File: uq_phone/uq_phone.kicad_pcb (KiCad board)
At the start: 4 copper layers, 116.9 x 105 mm, 170 parts, among them J1 USB4105-GF-A, J10 Conn_01x02, J11 FTSH-105-XX-X-DV, J12 Conn_ARM_SWD_TagConnect_TC2030, J2 S3B-PH-SM4-TB_LF__SN_, J3 20279-001E-03, J4 20279-001E-03, J5 KP15B-6S-SF_800_, J7 Conn_01x02, J8 541324562, J9 SJ-3551B-MSMT-TR-67, Q1 MMBT3904, Q2 MMBT3904, SW1 SKTAAAE010, SW2 SKTAAAE010, U1 MCP73871-2CCI_ML, U10 TPD3F303DQDR, U12 MCP1664T-E/OT, U14 TPD8F003DQDR, U15 TS3A5018RSVR, U16 NAU88C22YG, U2 TPS62162DSGR, U3 BQ27441DRZR-G1A, U4 RC7620_1104625, U5 TXB0108RGYR, U6 TXB0108RGYR, U7 STM32H730VBTx, U8 LSM6DSVTR, U9 DRV2603RUNR

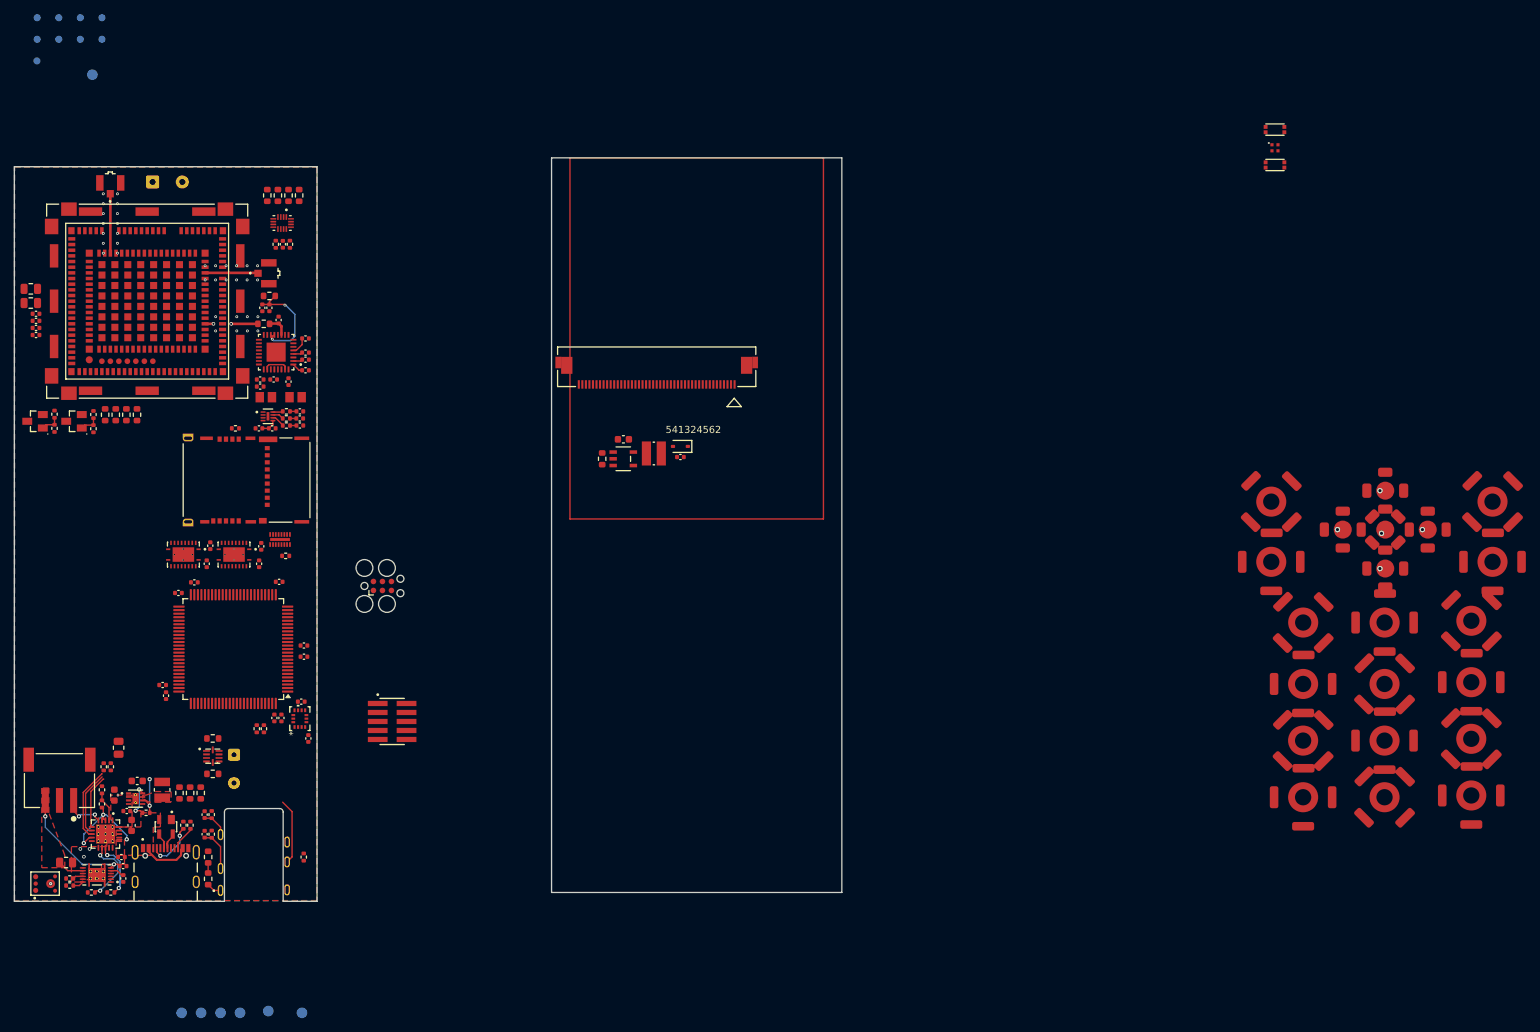
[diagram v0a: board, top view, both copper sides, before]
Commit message: Routing Init
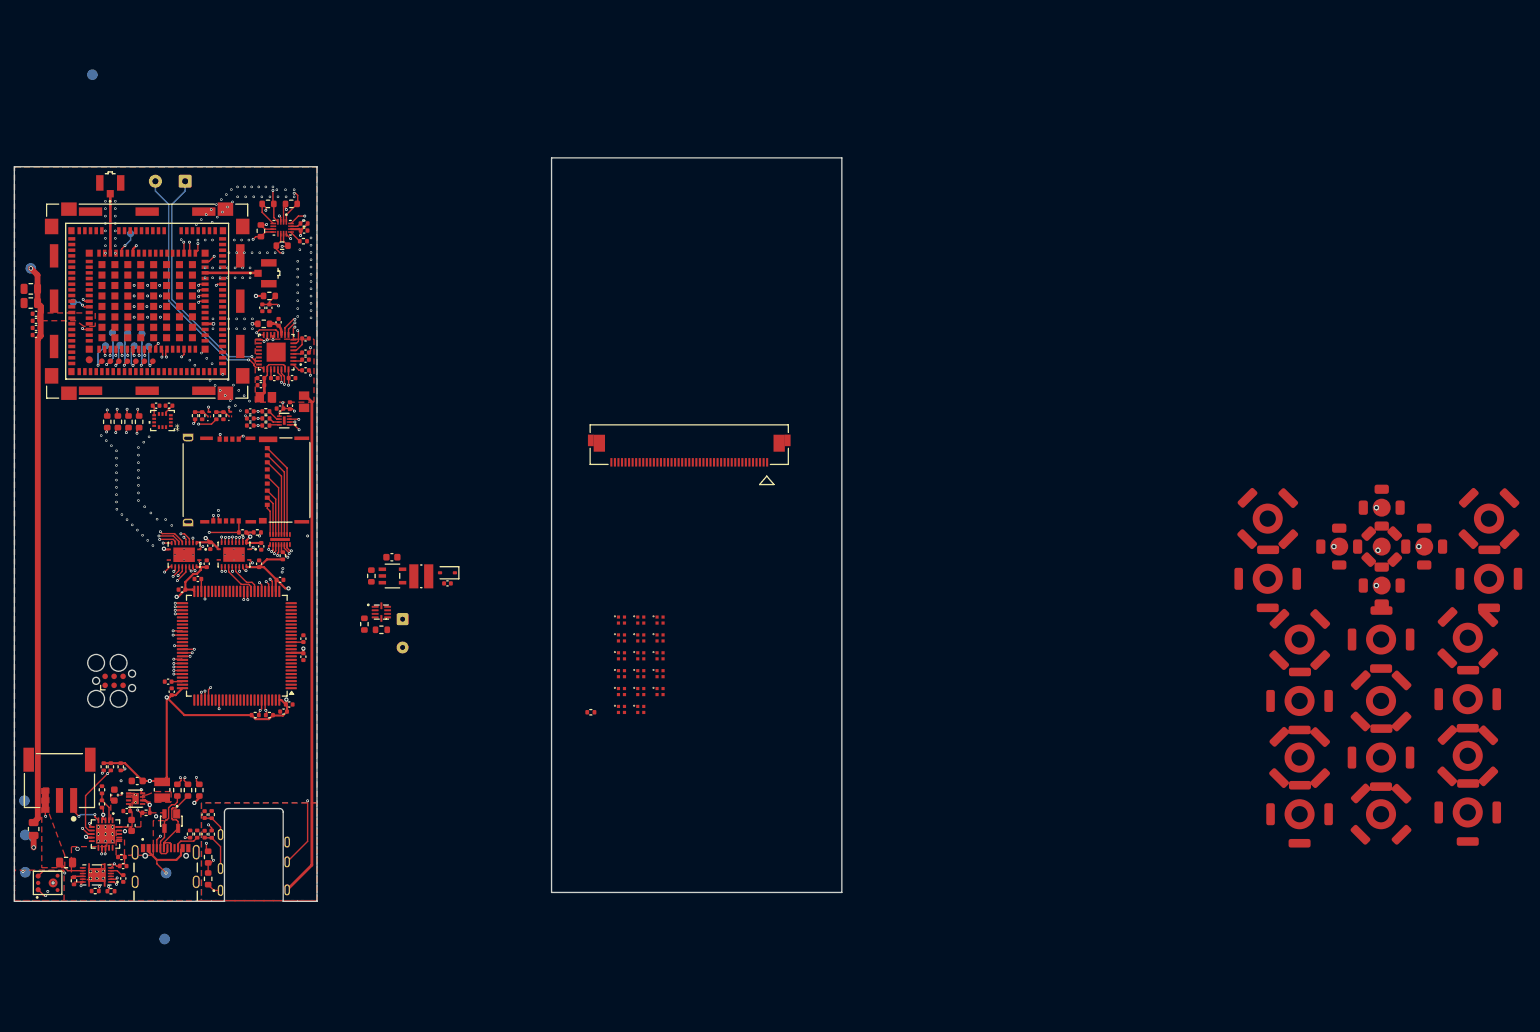
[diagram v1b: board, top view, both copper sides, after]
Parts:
- removed the J11 at (80.7, 146.6)
- removed the REF** at (209.4, 132.6)
- removed the REF** at (236.2, 115.5)
- removed the REF** at (209.4, 149.3)
- removed the REF** at (209.4, 157.3)
- removed the REF** at (209.4, 141.3)
- removed the REF** at (220.9, 149.3)
- removed the REF** at (204.9, 124.0)
- removed the REF** at (215.0, 119.5)
- removed the REF** at (221.0, 114.0)
- removed the REF** at (204.9, 115.5)
- removed the REF** at (220.9, 157.3)
- removed the REF** at (220.9, 141.3)
- removed the REF** at (221.0, 119.5)
- removed the REF** at (233.2, 157.1)
- removed the REF** at (227.0, 119.5)
- removed the REF** at (220.9, 132.6)
- removed the REF** at (233.2, 141.1)
- removed the REF** at (233.2, 132.4)
- removed the REF** at (236.2, 124.0)
- removed the REF** at (233.2, 149.1)
- removed the REF** at (221.0, 125.0)
- removed SW1, SW2: SKTAAAE010, custom_footprints:SKTAAAE010
- added LED10: XL-1010RGBC, custom_footprints:XL-1010RGBC-WS2812B, F.Cu at (115.4, 139.4)
- added LED11: XL-1010RGBC, custom_footprints:XL-1010RGBC-WS2812B, F.Cu at (115.4, 141.9)
- added LED12: XL-1010RGBC, custom_footprints:XL-1010RGBC-WS2812B, F.Cu at (115.4, 144.5)
- added LED13: XL-1010RGBC, custom_footprints:XL-1010RGBC-WS2812B, F.Cu at (118.2, 131.8)
- added LED14: XL-1010RGBC, custom_footprints:XL-1010RGBC-WS2812B, F.Cu at (118.2, 134.4)
- added LED15: XL-1010RGBC, custom_footprints:XL-1010RGBC-WS2812B, F.Cu at (118.2, 136.9)
- added LED16: XL-1010RGBC, custom_footprints:XL-1010RGBC-WS2812B, F.Cu at (118.2, 139.4)
- added LED17: XL-1010RGBC, custom_footprints:XL-1010RGBC-WS2812B, F.Cu at (118.2, 141.9)
- added LED2: XL-1010RGBC, custom_footprints:XL-1010RGBC-WS2812B, F.Cu at (112.7, 134.4)
- added LED3: XL-1010RGBC, custom_footprints:XL-1010RGBC-WS2812B, F.Cu at (112.7, 136.9)
- added LED4: XL-1010RGBC, custom_footprints:XL-1010RGBC-WS2812B, F.Cu at (112.7, 139.4)
- added LED5: XL-1010RGBC, custom_footprints:XL-1010RGBC-WS2812B, F.Cu at (112.7, 141.9)
- added LED6: XL-1010RGBC, custom_footprints:XL-1010RGBC-WS2812B, F.Cu at (112.7, 144.5)
- added LED7: XL-1010RGBC, custom_footprints:XL-1010RGBC-WS2812B, F.Cu at (115.4, 131.8)
- added LED8: XL-1010RGBC, custom_footprints:XL-1010RGBC-WS2812B, F.Cu at (115.4, 134.4)
- added LED9: XL-1010RGBC, custom_footprints:XL-1010RGBC-WS2812B, F.Cu at (115.4, 136.9)
- added R48: 330R, Resistor_SMD:R_0402_1005Metric, F.Cu at (108.8, 145.3)
- added REF**: 8.5mmSnaptron, custom_footprints:8.5mmSnaptron, F.Cu at (220.4, 151.7)
- added REF**: 8.5mmSnaptron, custom_footprints:8.5mmSnaptron, F.Cu at (232.7, 159.4)
- added REF**: 8.5mmSnaptron, custom_footprints:8.5mmSnaptron, F.Cu at (235.7, 118.0)
- added REF**: 8.5mmSnaptron, custom_footprints:8.5mmSnaptron, F.Cu at (232.7, 143.4)
- added REF**: 8.5mmSnaptron, custom_footprints:8.5mmSnaptron, F.Cu at (208.9, 151.7)
- added REF**: 8.5mmSnaptron, custom_footprints:8.5mmSnaptron, F.Cu at (204.4, 118.0)
- added REF**: 8.5mmSnaptron, custom_footprints:8.5mmSnaptron, F.Cu at (232.7, 151.4)
- added REF**: 6mmSnaptron, custom_footprints:6mmSnaptron, F.Cu at (220.5, 127.4)
- added REF**: 8.5mmSnaptron, custom_footprints:8.5mmSnaptron, F.Cu at (220.4, 135.0)
- added REF**: 6mmSnaptron, custom_footprints:6mmSnaptron, F.Cu at (226.5, 121.9)
- added REF**: 6mmSnaptron, custom_footprints:6mmSnaptron, F.Cu at (214.5, 121.9)
- added REF**: 8.5mmSnaptron, custom_footprints:8.5mmSnaptron, F.Cu at (204.4, 126.5)
- added REF**: 6mmSnaptron, custom_footprints:6mmSnaptron, F.Cu at (220.5, 116.4)
- added REF**: 8.5mmSnaptron, custom_footprints:8.5mmSnaptron, F.Cu at (208.9, 135.0)
- added REF**: 8.5mmSnaptron, custom_footprints:8.5mmSnaptron, F.Cu at (220.4, 159.7)
- added REF**: 6mmSnaptron, custom_footprints:6mmSnaptron, F.Cu at (220.5, 121.9)
- added REF**: 8.5mmSnaptron, custom_footprints:8.5mmSnaptron, F.Cu at (220.4, 143.7)
- added REF**: 8.5mmSnaptron, custom_footprints:8.5mmSnaptron, F.Cu at (232.7, 134.8)
- added REF**: 8.5mmSnaptron, custom_footprints:8.5mmSnaptron, F.Cu at (208.9, 143.7)
- added REF**: 8.5mmSnaptron, custom_footprints:8.5mmSnaptron, F.Cu at (208.9, 159.7)
- added REF**: 8.5mmSnaptron, custom_footprints:8.5mmSnaptron, F.Cu at (235.7, 126.5)
- LED1: value XINGLIGHT XL-1010RGBC-WS2812B -> XL-1010RGBC
- Q1, Q2: value MMBT3904 -> MMBT3904LP-7; footprint MMBT3904LT1G:SOT95P240X111-3N -> MMBT3904LP-7:DFN101X61X53-3N
- moved LED1 113.9 mm to (112.7, 131.8)
- moved TP6 111.9 mm to (29.7, 82.6)
- moved C27 51.0 mm to (49.2, 102.0), turned to 180 degrees
- moved C28 46.6 mm to (47.4, 102.0), turned to 0 degrees
- moved TP10 46.5 mm to (40.2, 93.5)
- moved U8 46.4 mm to (48.3, 104.1), turned to 180 degrees
- moved R45 46.3 mm to (61.7, 119.9), turned to 180 degrees
- moved TP12 44.8 mm to (42.3, 93.5)
- moved TP11 44.5 mm to (41.2, 91.7)
- moved TP14 44.0 mm to (44.3, 93.5)
- moved TP16 43.3 mm to (46.4, 93.6)
- moved TP2 42.7 mm to (28.8, 157.8)
- moved TP13 42.6 mm to (43.4, 91.8)
- moved TP15 42.0 mm to (45.4, 91.8)
- moved TP9 40.3 mm to (35.7, 87.4)
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- renumbered C15 to C10, C16 to C11, C17 to C12, C18 to C13, C19 to C14, C20 to C15, C21 to C16, C22 to C17, C23 to C18, C24 to C19, C25 to C20, C26 to C21, C27 to C22, C28 to C23, C29 to C24, C30 to C25, C31 to C26, C32 to C27, C33 to C28, C8 to C29, C9 to C30, C10 to C31, C11 to C32, C12 to C33, C48 to C34, C49 to C35, C50 to C36, C35 to C37, C36 to C38, C37 to C39, C38 to C40, C39 to C41, C56 to C42, C47 to C43, C40 to C44, C41 to C45, C42 to C46, C43 to C47, C44 to C48, C45 to C49, C7 to C6, C6 to C7, C13 to C8, C14 to C9, D5 to D2, J9 to J10, J10 to J11, J12 to J6, J5 to J8, J8 to J9, MK2 to MK1, R8 to R10, R39 to R23, R26 to R24, R27 to R25, R28 to R26, R29 to R27, R30 to R28, R31 to R29, R23 to R30, R24 to R31, R25 to R32, R32 to R33, R38 to R34, R40 to R35, R41 to R36, R42 to R37, R47 to R38, R48 to R39, R43 to R40, R44 to R41, R45 to R42, R46 to R43, R49 to R44, R50 to R45, R51 to R46, R54 to R47, R9 to R8, R10 to R9, U14 to U11, U15 to U13, U16 to U14
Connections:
- C41 pad 1: unconnected-(C39-Pad1) -> Net-(U14-RMICN)
- C42 pad 1: (no net) -> Net-(MK1-OUTPUT)
- C48 pad 1: unconnected-(C44-Pad1) -> Net-(U14-VREF)
- D1 pad 3: USB_P -> USB_N
- D1 pad 4: USB_N -> USB_P
- LED1 pad 1: unconnected-(LED1-DO-Pad1) -> Net-(LED1-DO)
- LED1 pad 2: unconnected-(LED1-VDD-Pad2) -> +3.3V
- LED1 pad 3: unconnected-(LED1-GND-Pad3) -> GND
- LED1 pad 4: unconnected-(LED1-DI-Pad4) -> Net-(LED1-DI)
- MK1 pad 1: (no net) -> Net-(MK1-OUTPUT)
- R35 pad 1: AUD_SW -> AUD_SW_L
- R36 pad 2: unconnected-(R41-Pad2) -> Net-(U13-~{EN})
- U13 pad 13: unconnected-(R41-Pad2) -> Net-(U13-~{EN})
- U13 pad 15: AUD_SW -> AUD_SW_L
- U13 pad 9: MCU_AUD_IN -> unconnected-(U13-NC3-Pad9)
- U14 pad 19: (no net) -> unconnected-(U14-LAUXIN-Pad19)
- U14 pad 20: (no net) -> unconnected-(U14-RAUXIN-Pad20)
- U14 pad 21: (no net) -> unconnected-(U14-AUXOUT1-Pad21)
- U14 pad 22: (no net) -> unconnected-(U14-AUXOUT2-Pad22)
- U14 pad 27: unconnected-(C44-Pad1) -> Net-(U14-VREF)
- U14 pad 3: (no net) -> unconnected-(U14-LLIN/GPIO2-Pad3)
- U14 pad 5: unconnected-(C39-Pad1) -> Net-(U14-RMICN)
- U14 pad 6: (no net) -> unconnected-(U14-RLIN/GPIO3-Pad6)
- U4 pad 38: MOB_GNSS_ANT -> unconnected-(U4A-RF_GNSS-Pad38)
- U4 pad P1: (no net) -> GND
- U4 pad P10: (no net) -> GND
- U4 pad P11: (no net) -> GND
- U4 pad P12: (no net) -> GND
- U4 pad P13: (no net) -> GND
- U4 pad P14: (no net) -> GND
- U4 pad P15: (no net) -> GND
- U4 pad P16: (no net) -> GND
- U4 pad P17: (no net) -> GND
- U4 pad P18: (no net) -> GND
- U4 pad P19: (no net) -> GND
- U4 pad P2: (no net) -> GND
- U4 pad P20: (no net) -> GND
- U4 pad P3: (no net) -> GND
- U4 pad P4: (no net) -> GND
- U4 pad P5: (no net) -> GND
- U4 pad P6: (no net) -> GND
- U4 pad P7: (no net) -> GND
- U4 pad P8: (no net) -> GND
- U4 pad P9: (no net) -> GND
- U5 pad 1: MOB_DTR -> MOB_DSR
- U5 pad 12: MCU_DSR -> MCU_RI
- U5 pad 16: MCU_RI -> MCU_RXD
- U5 pad 17: MCU_DCD -> MCU_DTR
- U5 pad 18: MCU_RXD -> MCU_DCD
- U5 pad 20: MCU_DTR -> MCU_DSR
- U5 pad 3: MOB_RXD -> MOB_DCD
- U5 pad 4: MOB_DCD -> MOB_DTR
- U5 pad 5: MOB_RI -> MOB_RXD
- U5 pad 9: MOB_DSR -> MOB_RI
- U6 pad 12: AUD_SW_H -> MCU_AUD_OUT_L_H
- U6 pad 13: MCU_AUD_SYNC_H -> MCU_AUD_BCLK_H
- U6 pad 14: MCU_AUD_BCLK_H -> AUD_SW_H
- U6 pad 15: MCU_AUD_OUT_L_H -> MCU_AUD_SYNC_H
- U6 pad 6: MCU_AUD_OUT_L -> MCU_AUD_SYNC_L
- U6 pad 7: MCU_AUD_BCLK_L -> AUD_SW_L
- U6 pad 8: MCU_AUD_SYNC_L -> MCU_AUD_BCLK_L
- U6 pad 9: AUD_SW_L -> MCU_AUD_OUT_L
- U7 pad 35: unconnected-(U7-PB1-Pad35) -> MOB_WAKE_H
- U7 pad 36: unconnected-(U7-PB2-Pad36) -> MOB_PWR_CTL
- U7 pad 47: unconnected-(U7-PB11-Pad47) -> MOB_RST_CTL
- U7 pad 59: MCU_DTR -> MCU_DCD
- U7 pad 60: MCU_DCD -> MCU_DTR
- U7 pad 91: MOB_RST_CTL -> unconnected-(U7-PB5-Pad91)
- U7 pad 92: MOB_WAKE_H -> unconnected-(U7-PB6-Pad92)
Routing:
- net +1.8V: track 0.00 -> 112.0 mm, vias 0 -> 6
- net Net-(MK1-OUTPUT): track 0.00 -> 110.4 mm, vias 0 -> 2
- net +3.3V: track 6.14 -> 111.2 mm, vias 2 -> 7
- net AGND: track 0.00 -> 99.7 mm, vias 0 -> 3
- net HP_DET: track 9.27 -> 90.3 mm, vias 0 -> 5
- net Net-(C37-Pad2): track 1.43 -> 81.5 mm, vias 0 -> 2
- net +VMOB: track 0.00 -> 80.0 mm, vias 0 -> 1
- net SDA: track 0.00 -> 64.0 mm, vias 0 -> 4
- net SCL: track 0.00 -> 63.4 mm, vias 0 -> 4
- net Net-(U4A-USB_VBUS): track 0.00 -> 63.0 mm, vias 0 -> 2
- net /Mobile/MOB_USB_N: track 0.00 -> 63.0 mm, vias 0 -> 2
- net /Mobile/MOB_USB_P: track 0.00 -> 62.9 mm, vias 0 -> 2
- net FUEL_GPO: track 1.56 -> 56.6 mm, vias 0 -> 3
- net MCU_AUD_SYNC_L: track 0.00 -> 53.1 mm, vias 0 -> 2
- net MCU_AUD_BCLK_L: track 0.00 -> 53.1 mm, vias 0 -> 2
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- added copper zone on F.Cu, net +VMOB
- added copper zone on B.Cu, net AGND
- added copper zone on F.Cu, net AGND
- added copper zone on In2.Cu, net GND
